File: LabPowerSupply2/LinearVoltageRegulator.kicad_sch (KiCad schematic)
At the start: 16 parts, among them Q1_LVR1 PJA3404_R1_00001, Q2_LVR1 PJA3404_R1_00001, Q3_LVR1 PJA3404_R1_00001, Q4_LVR1 PJA3404_R1_00001

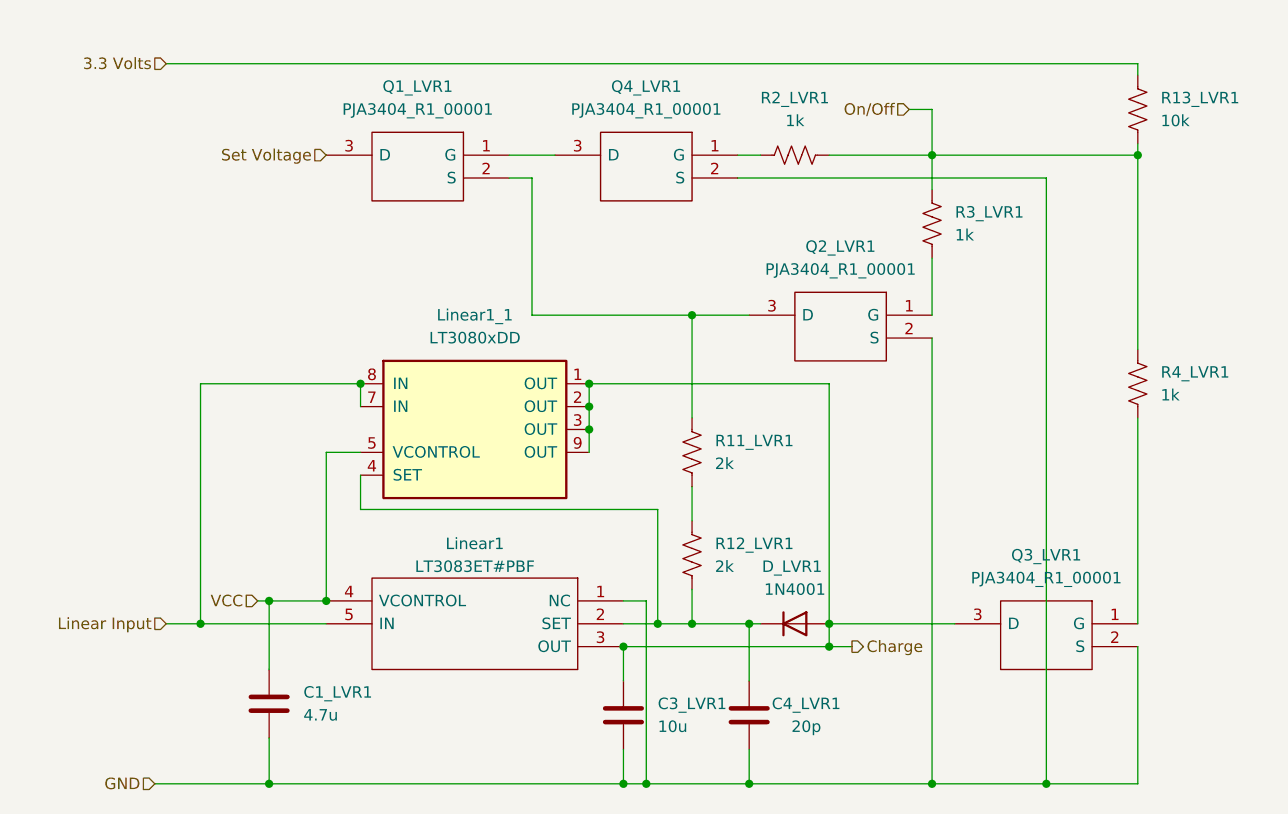
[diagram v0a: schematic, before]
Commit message: Beautifing the Schematic
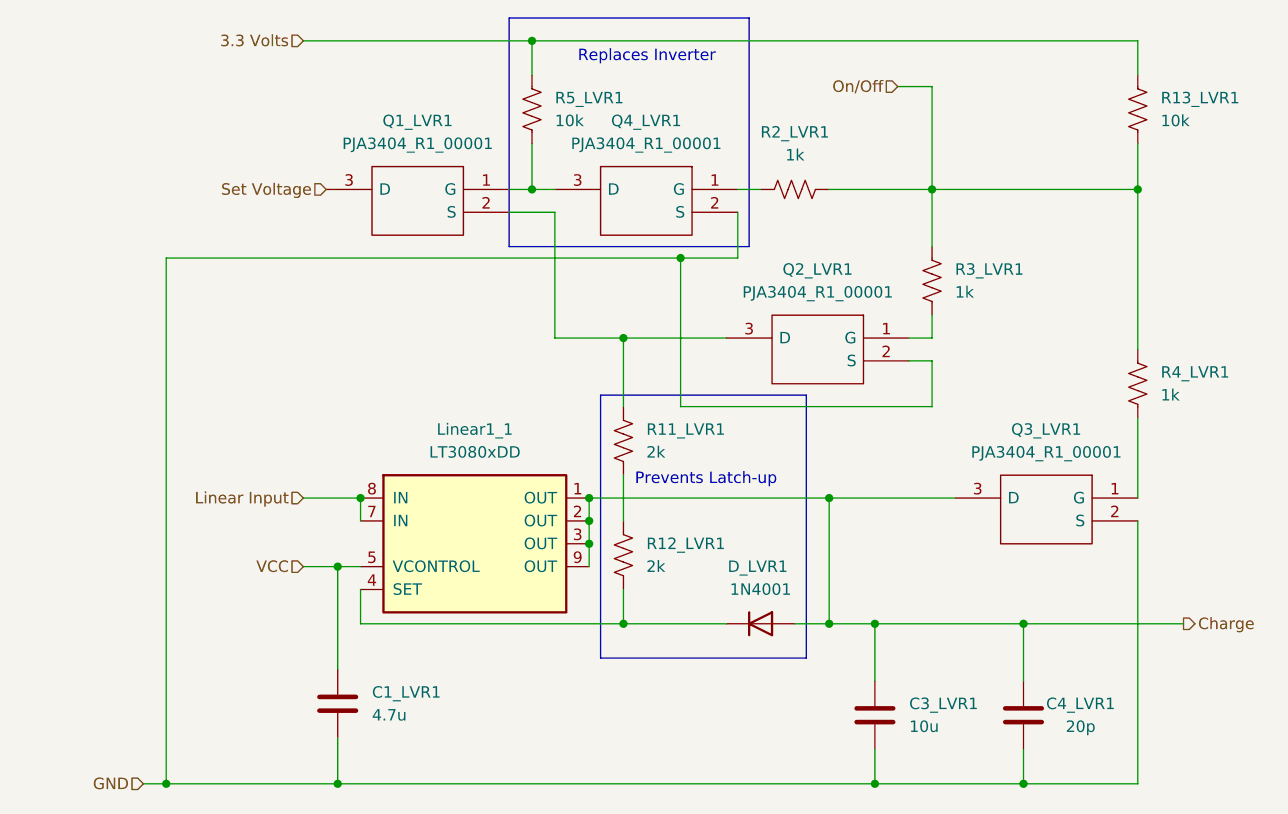
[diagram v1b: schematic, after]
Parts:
- removed Linear1: LT3083ET#PBF, SamacSys_Parts:TO170P457X1022X2306-5P, symbol SamacSys_Parts:LT3083ET#PBF
- added R5_LVR1: 10k, symbol Device:R_US
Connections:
- net 3.3 Volts: now also R5_LVR1.1
- net Charge: now also C4_LVR1.1
- net at D_LVR1.1 (K), Linear1_1.4 (SET), R12_LVR1.1: no longer C4_LVR1.1
- net at Q1_LVR1.1 (G), Q4_LVR1.3 (D): now also R5_LVR1.2
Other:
- note added: "Prevents Latch-up"
- note added: "Replaces Inverter"
- moved on the sheet: C1_LVR1, C3_LVR1, C4_LVR1, D_LVR1, Linear1_1, Q1_LVR1, Q2_LVR1, Q3_LVR1, Q4_LVR1, R11_LVR1, R12_LVR1, R2_LVR1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
